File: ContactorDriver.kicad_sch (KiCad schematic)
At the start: 20 parts, among them Con1 LED, Con3 LED, J4 Conn_01x04, J6 Conn_01x04, Q4 IRLML0030, Q6 IRLML0030, U4 TCMT1106, U5 TCMT1106

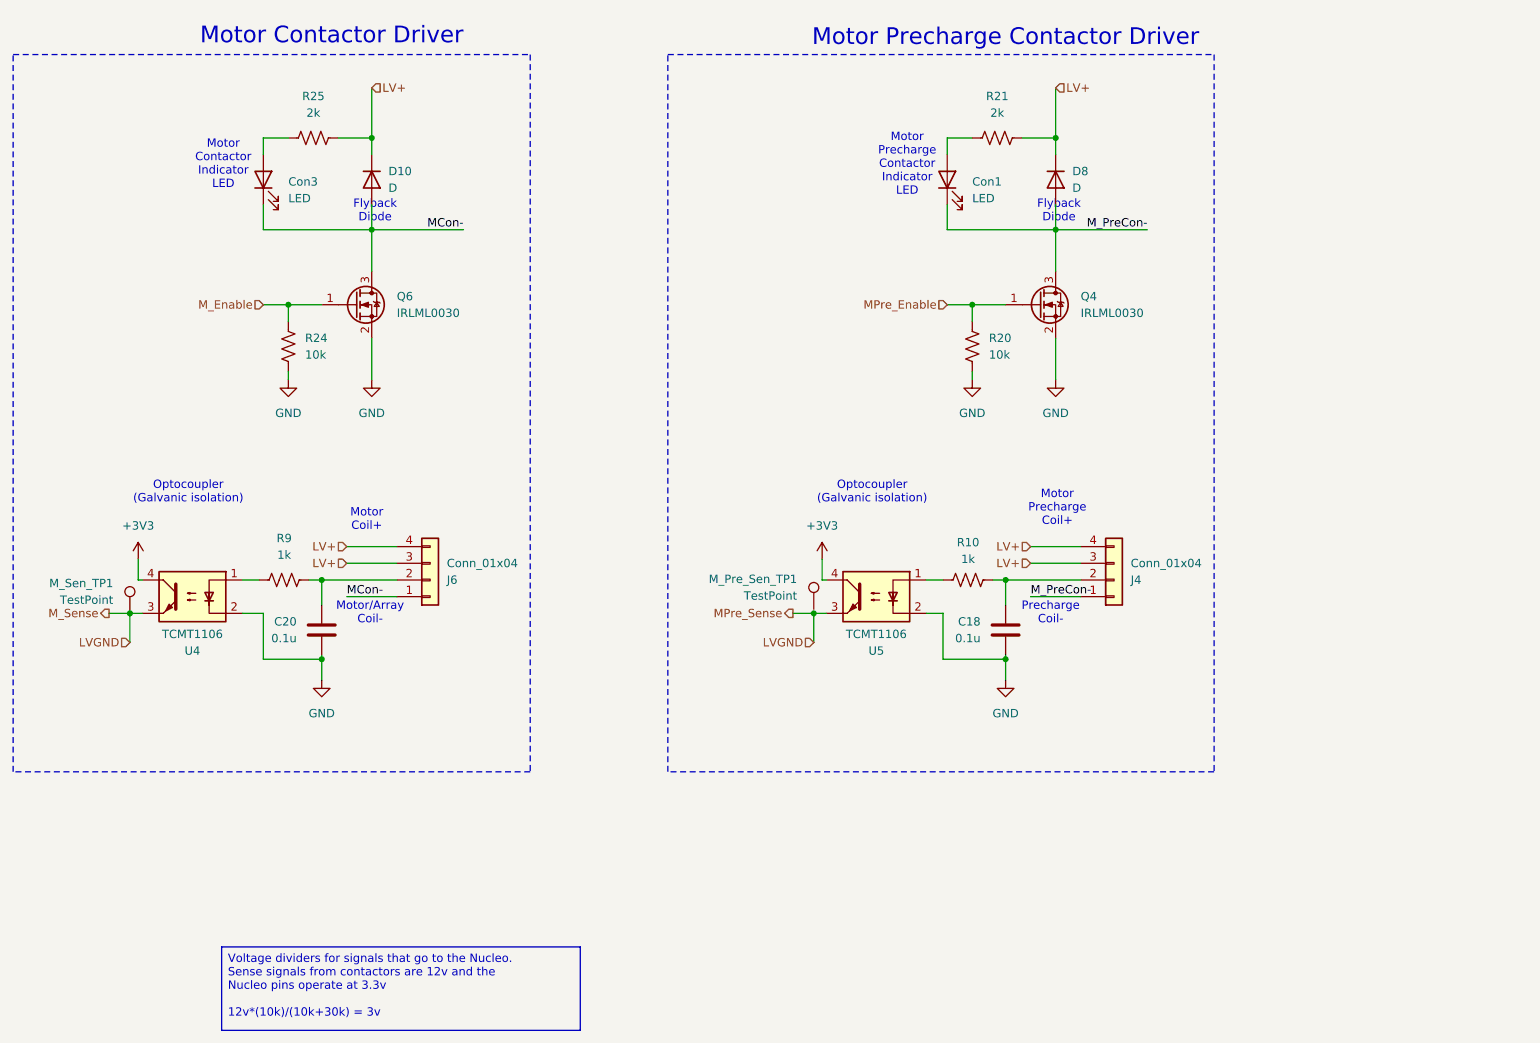
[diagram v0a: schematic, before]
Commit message: layout start
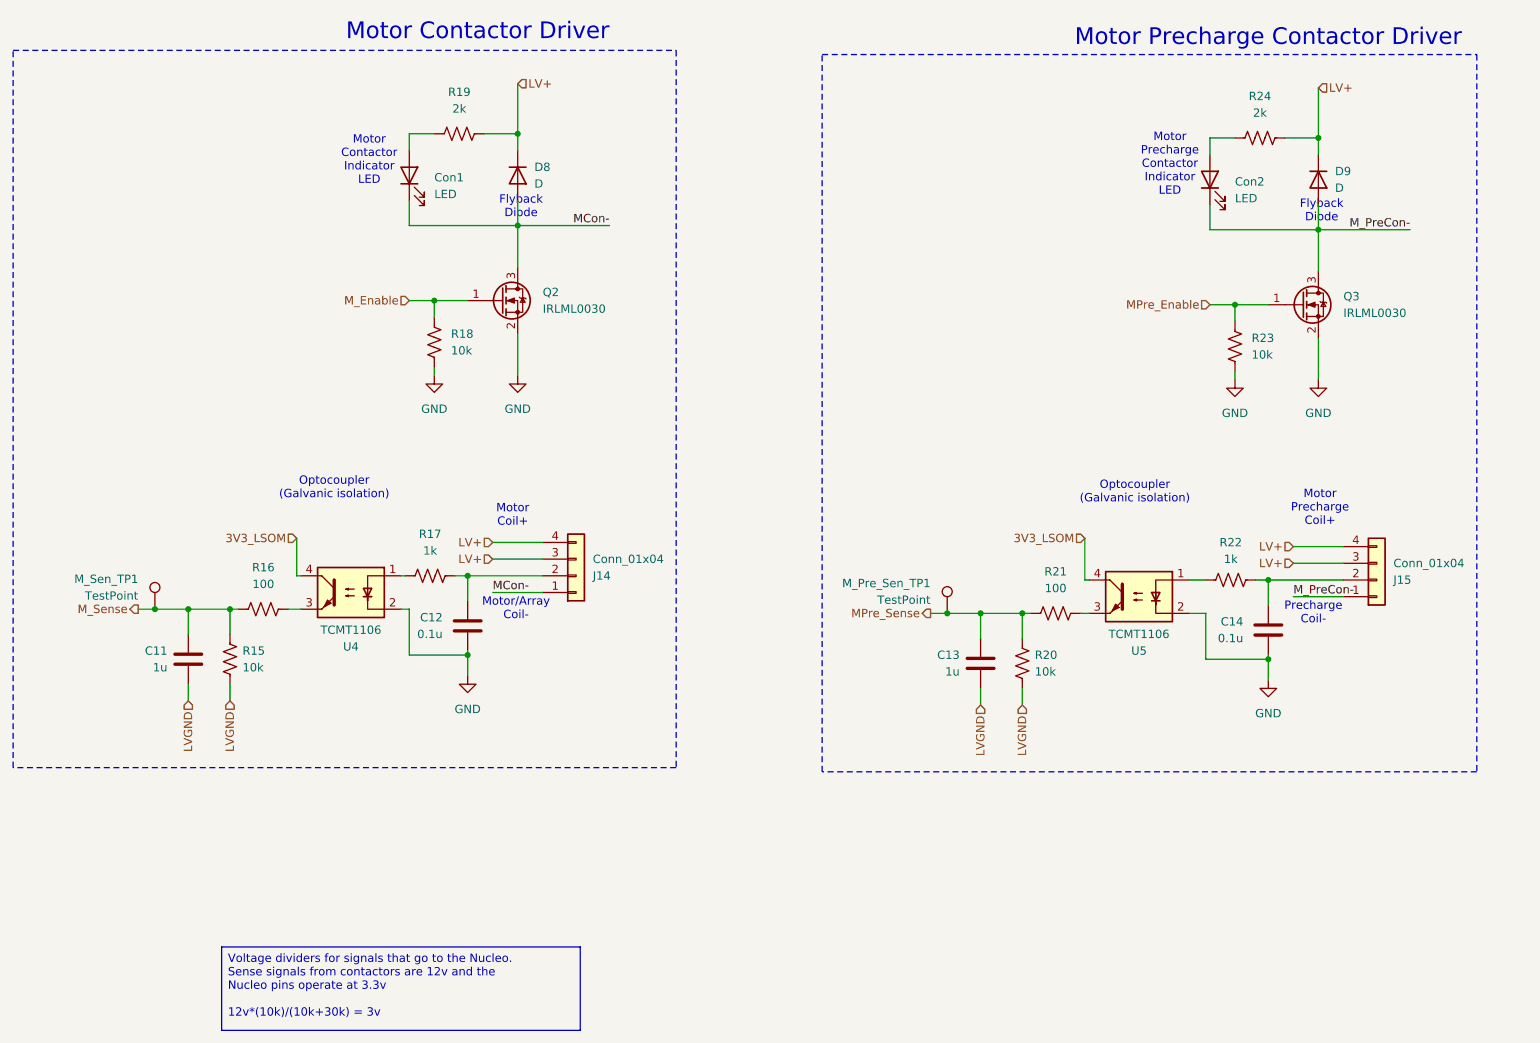
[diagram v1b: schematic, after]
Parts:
- added C11, C13: 1u, Capacitor_SMD:C_0805_2012Metric, symbol Device:C
- added R15, R20: 10k, Resistor_SMD:R_0805_2012Metric, symbol Device:R_US
- added R16, R21: 100, Resistor_SMD:R_0805_2012Metric, symbol Device:R_US
- J14: renamed from J6; footprint utsvt-conn:Molex_MicroFit3.0_1x4xP3.00mm_PolarizingPeg_Vertical -> utsvt_conn:Molex_MicroFit3.0_1x4xP3.00mm_PolarizingPeg_Vertical
- J15: renamed from J4; footprint utsvt-conn:Molex_MicroFit3.0_1x4xP3.00mm_PolarizingPeg_Vertical -> utsvt_conn:Molex_MicroFit3.0_1x4xP3.00mm_PolarizingPeg_Vertical
- M_Pre_Sen_TP1, M_Sen_TP1: footprint utsvt-special:TestPoint_HEX_3mmID -> UTSVT_Special:TestPoint_HEX_3mmID
- renumbered C20 to C12, C18 to C14, Con3 to Con1, Con1 to Con2, D10 to D8, D8 to D9, Q6 to Q2, Q4 to Q3, R9 to R17, R24 to R18, R25 to R19, R10 to R22, R20 to R23, R21 to R24
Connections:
- net LVGND: now also C11.1, C13.1, R15.2, R20.2; no longer M_Sen_TP1.1, U4.3, U5.3
- net MPre_Sense: now reaches M_Pre_Sen_TP1.1
- net MPre_Sense: now also C13.2, R20.1, R21.1
- net +3V3 renamed 3V3_LSOM
- new net: R21.2, U5.3
- new net: R16.2, U4.3
- new net M_Sense: C11.2, M_Sen_TP1.1, R15.1, R16.1
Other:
- moved on the sheet: C12, C14, Con1, Con2, D8, D9, J14, J15, M_Sen_TP1, Q2, Q3, R17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
